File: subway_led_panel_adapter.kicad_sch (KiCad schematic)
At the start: 28 parts, among them J1 Conn_02x06_Odd_Even, J2 Conn_02x10_Odd_Even, J3 Conn_02x06_Odd_Even, J4 Conn_02x20_Odd_Even, U1 74AHCT244, U2 ChinaBluePill, U3 74LVC1G123

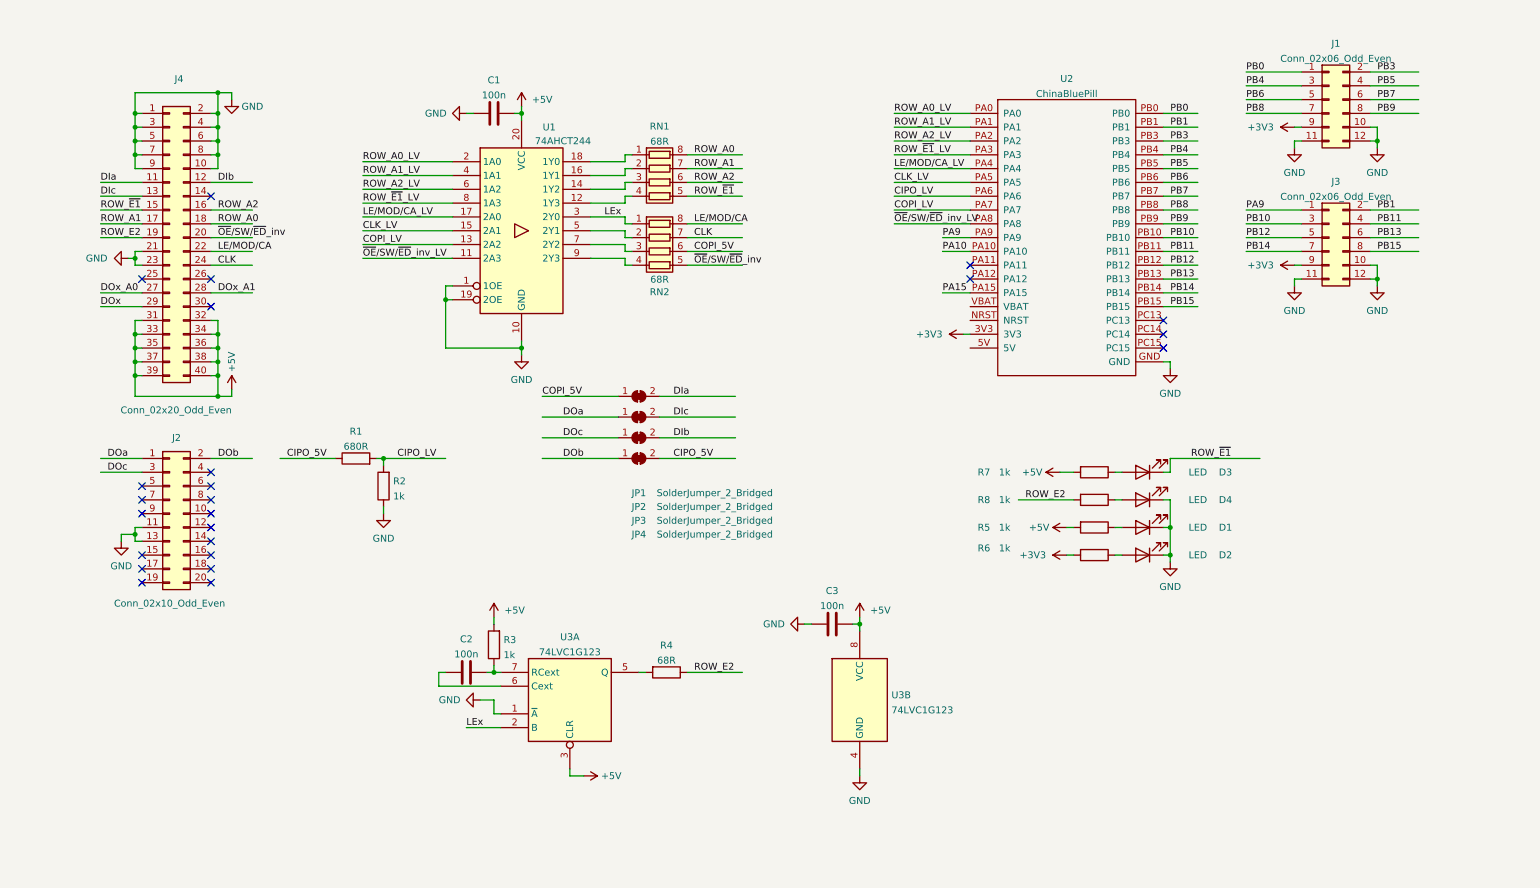
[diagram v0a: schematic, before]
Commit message: more work
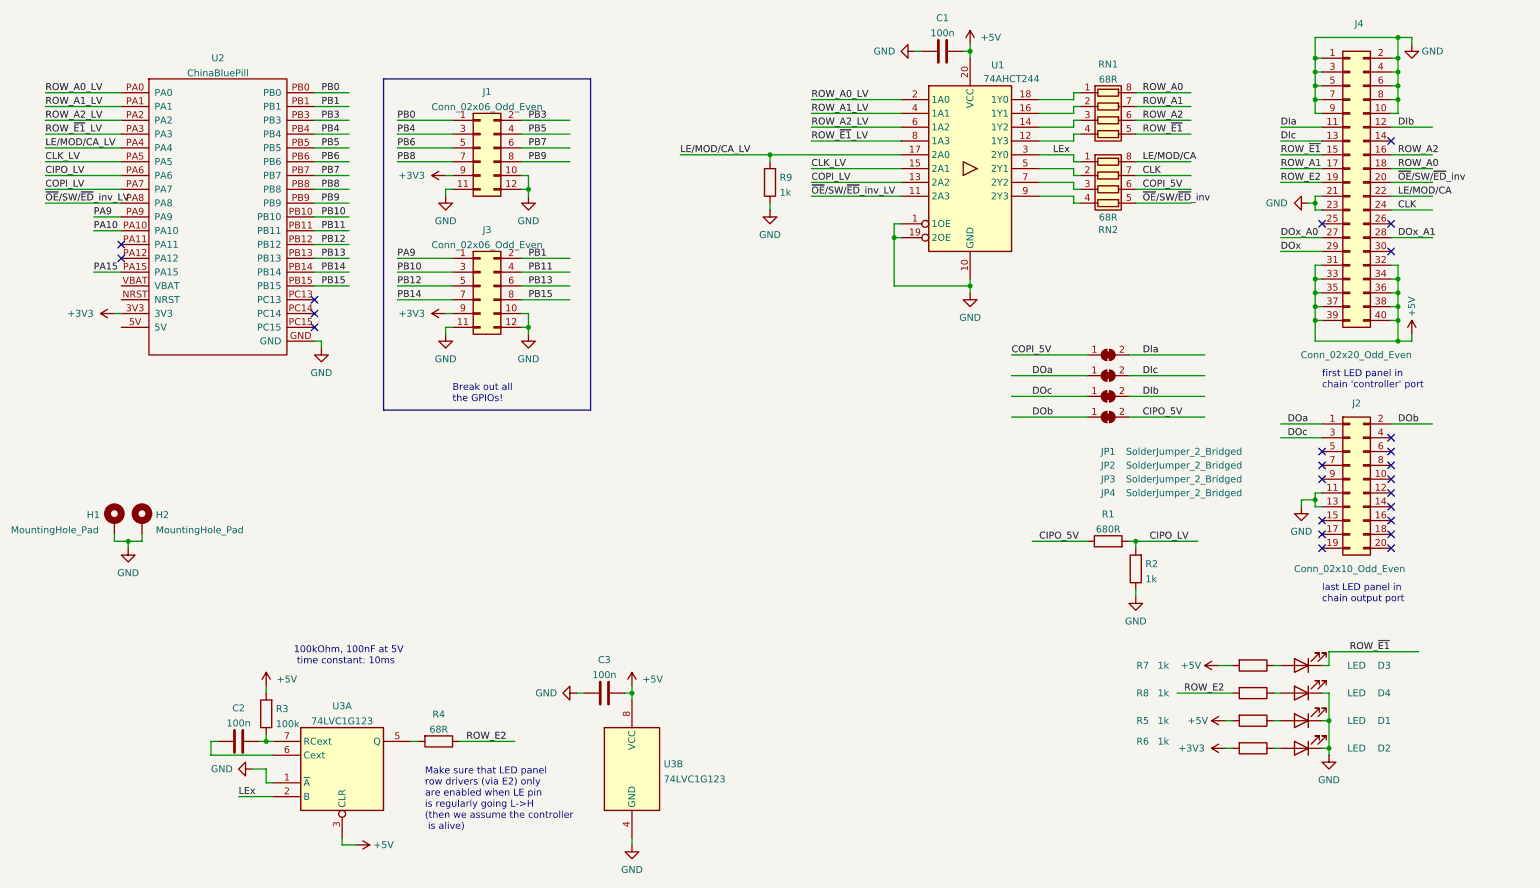
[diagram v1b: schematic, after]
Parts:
- added H1, H2: MountingHole_Pad, MountingHole:MountingHole_3.2mm_M3_Pad, symbol Mechanical:MountingHole_Pad
- added R9: 1k, Resistor_SMD:R_0603_1608Metric, symbol Device:R
- R3: value 1k -> 100k
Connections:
- net GND: now also H1.1, H2.1, R9.1
- net LE/MOD/CA_LV: now also R9.2
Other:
- note added: "100kOhm, 100nF at 5V time constant: 10ms"
- note added: "Break out all the GPIOs!"
- note added: "Make sure that LED panel row drivers (via E2) only are enabled when LE pin is regularly going L->H (then we assume the controller is alive)"
- note added: "first LED panel in chain 'controller' port"
- note added: "last LED panel in chain output port"
- moved on the sheet: C1, C2, C3, D1, D2, D3, D4, J1, J2, J3, J4, JP1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
